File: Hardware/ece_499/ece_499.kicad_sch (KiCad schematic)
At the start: 44 parts, among them J1 Conn_01x04, J2 Conn_01x04, J3 Conn_01x04, J4 Conn_01x04, J5 Conn_01x04, Q1 DMN2004WK, Q2 DMN2004WK, Q3 DMN2004WK, Q4 DMN2004WK, SW1 RotaryEncoder_Switch, U1 Xiao ESP32-C3, U2 ATA6561-GAQW-N, U3 AP62200WU-7, U4 I2C_LCD

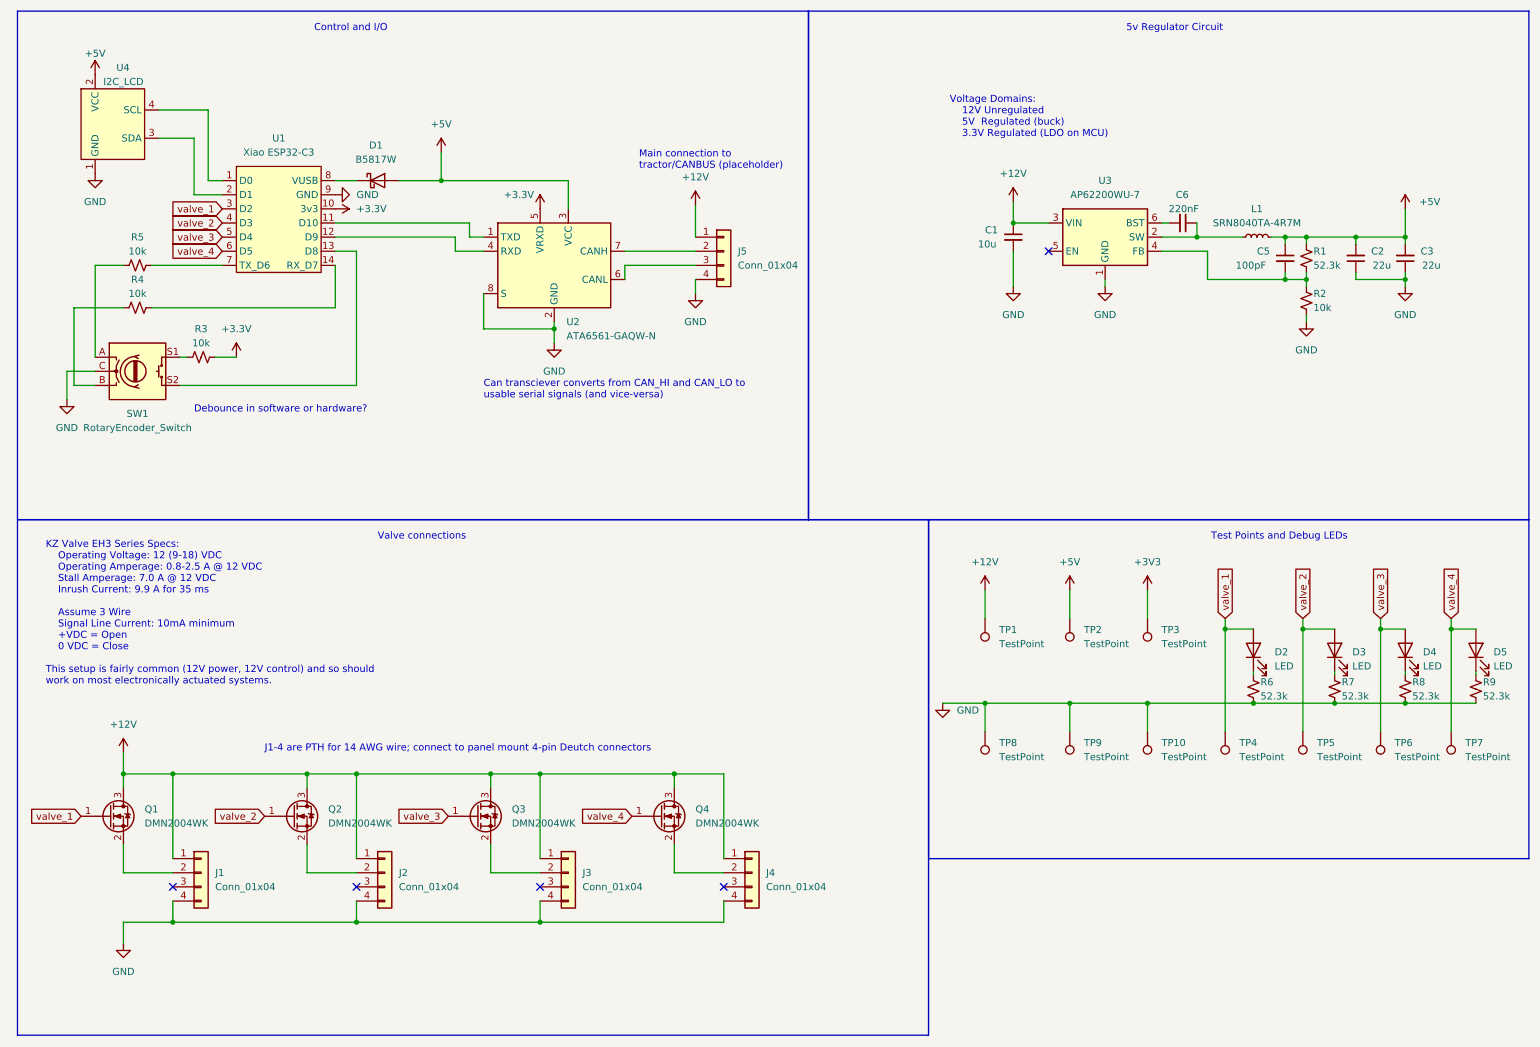
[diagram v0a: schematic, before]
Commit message: Cursed debouncy :(
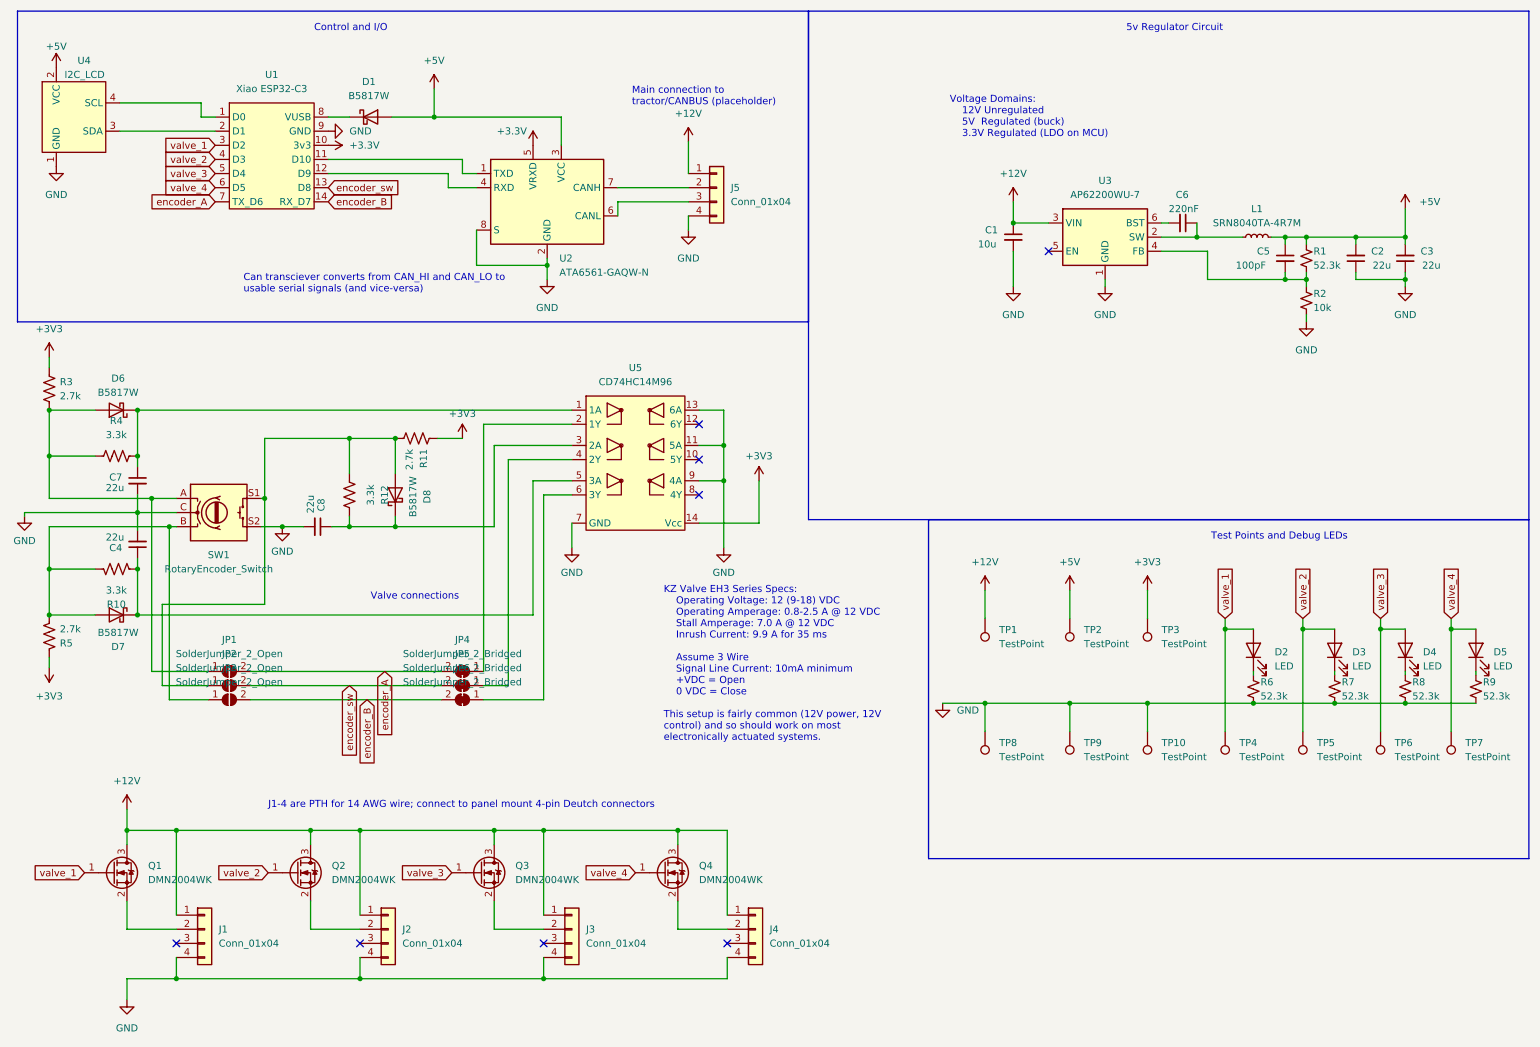
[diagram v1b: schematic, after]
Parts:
- removed R3, R4, R5: 10k, Resistor_SMD:R_1206_3216Metric_Pad1.30x1.75mm_HandSolder, symbol Device:R_Small_US
- added C4, C7, C8: 22u, Capacitor_SMD:C_0805_2012Metric_Pad1.18x1.45mm_HandSolder, symbol Device:C_Small
- added D6, D7, D8: B5817W, Diode_SMD:D_SOD-123, symbol Diode:1N5817
- added JP1, JP2, JP3: SolderJumper_2_Open, symbol Jumper:SolderJumper_2_Open
- added JP4, JP5, JP6: SolderJumper_2_Bridged, symbol Jumper:SolderJumper_2_Bridged
- added R10, R12, R4: 3.3k, symbol Device:R_US
- added R11, R3, R5: 2.7k, symbol Device:R_US
- added U5: CD74HC14M96, Package_SO:SO-14_3.9x8.65mm_P1.27mm, symbol Imported_Parts:CD74HC14M96
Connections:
- net +3V3: now also R11.1, R3.1, R5.1, U5.14 (Vcc)
- net GND: now also SW1.S2, C4.2, C7.2, C8.2, U5.11 (5A), U5.13 (6A), U5.7 (GND), U5.9 (4A)
- net at SW1.A: now also D6.2 (A), JP1.1 (A), R3.2, R4.2
- net encoder_A: now reaches U1.7 (TX_D6)
- net encoder_A: now also JP1.2 (B), JP4.2 (B)
- net at SW1.S1: now also D8.2 (A), JP2.1 (A), R11.2, R12.2
- net encoder_sw: now reaches U1.13 (D8)
- net encoder_sw: now also JP2.2 (B), JP5.2 (B); no longer SW1.S2
- net encoder_B: now reaches U1.14 (RX_D7)
- net encoder_B: now also JP3.2 (B), JP6.2 (B)
- net at SW1.B: now also D7.2 (A), JP3.1 (A), R10.2, R5.2
- new net: JP4.1 (A), U5.2 (1Y)
- new net: JP5.1 (A), U5.4 (2Y)
- new net: C7.1, D6.1 (K), R4.1, U5.1 (1A)
- new net: C8.1, D8.1 (K), R12.1, U5.3 (2A)
- new net: C4.1, D7.1 (K), R10.1, U5.5 (3A)
- new net: JP6.1 (A), U5.6 (3Y)
- no-connect marks 5 -> 8
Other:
- note removed: "Debounce in software or hardware?"
- moved on the sheet: D1, J1, J2, J3, J4, J5, Q1, Q2, Q3, Q4, SW1, U1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
